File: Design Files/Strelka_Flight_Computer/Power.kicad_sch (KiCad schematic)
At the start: 41 parts, among them J1 1S_LiPo_LARGE_HOLE_XT-30, Q1 ??, Q2 ??, SW3 SW_DIP_x01, U16 TPS61085DGKR, U2 AP9101CK6, U3 AMS1117-3.3

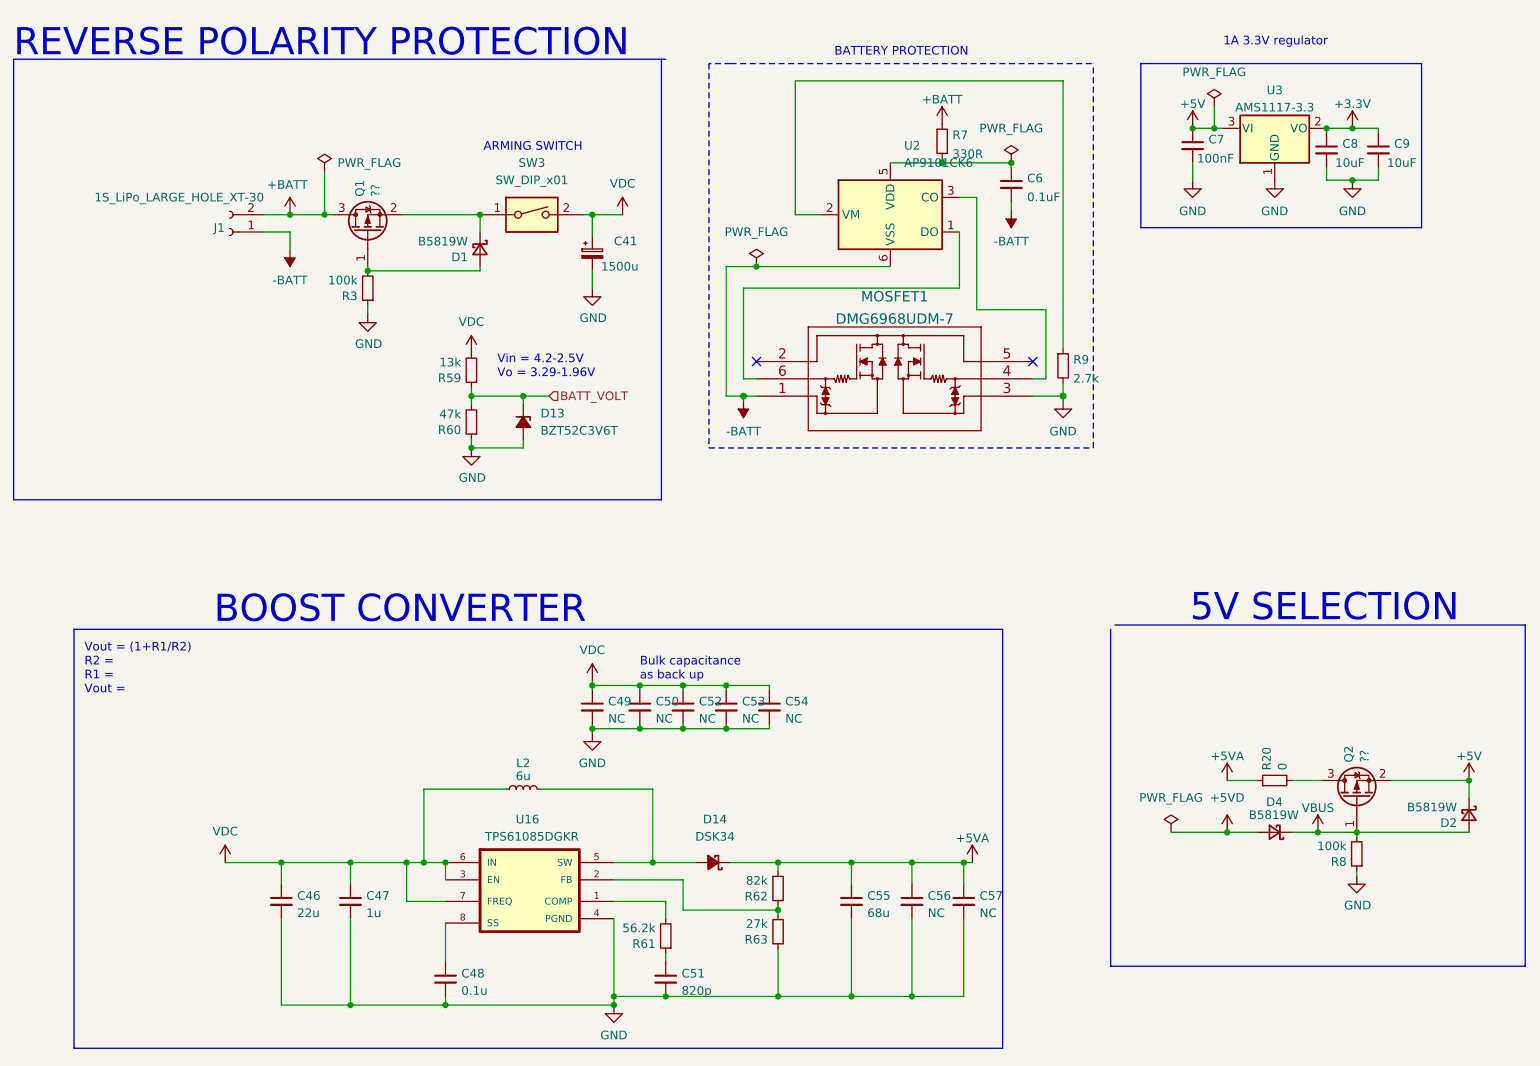
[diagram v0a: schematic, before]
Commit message: Creating BOM
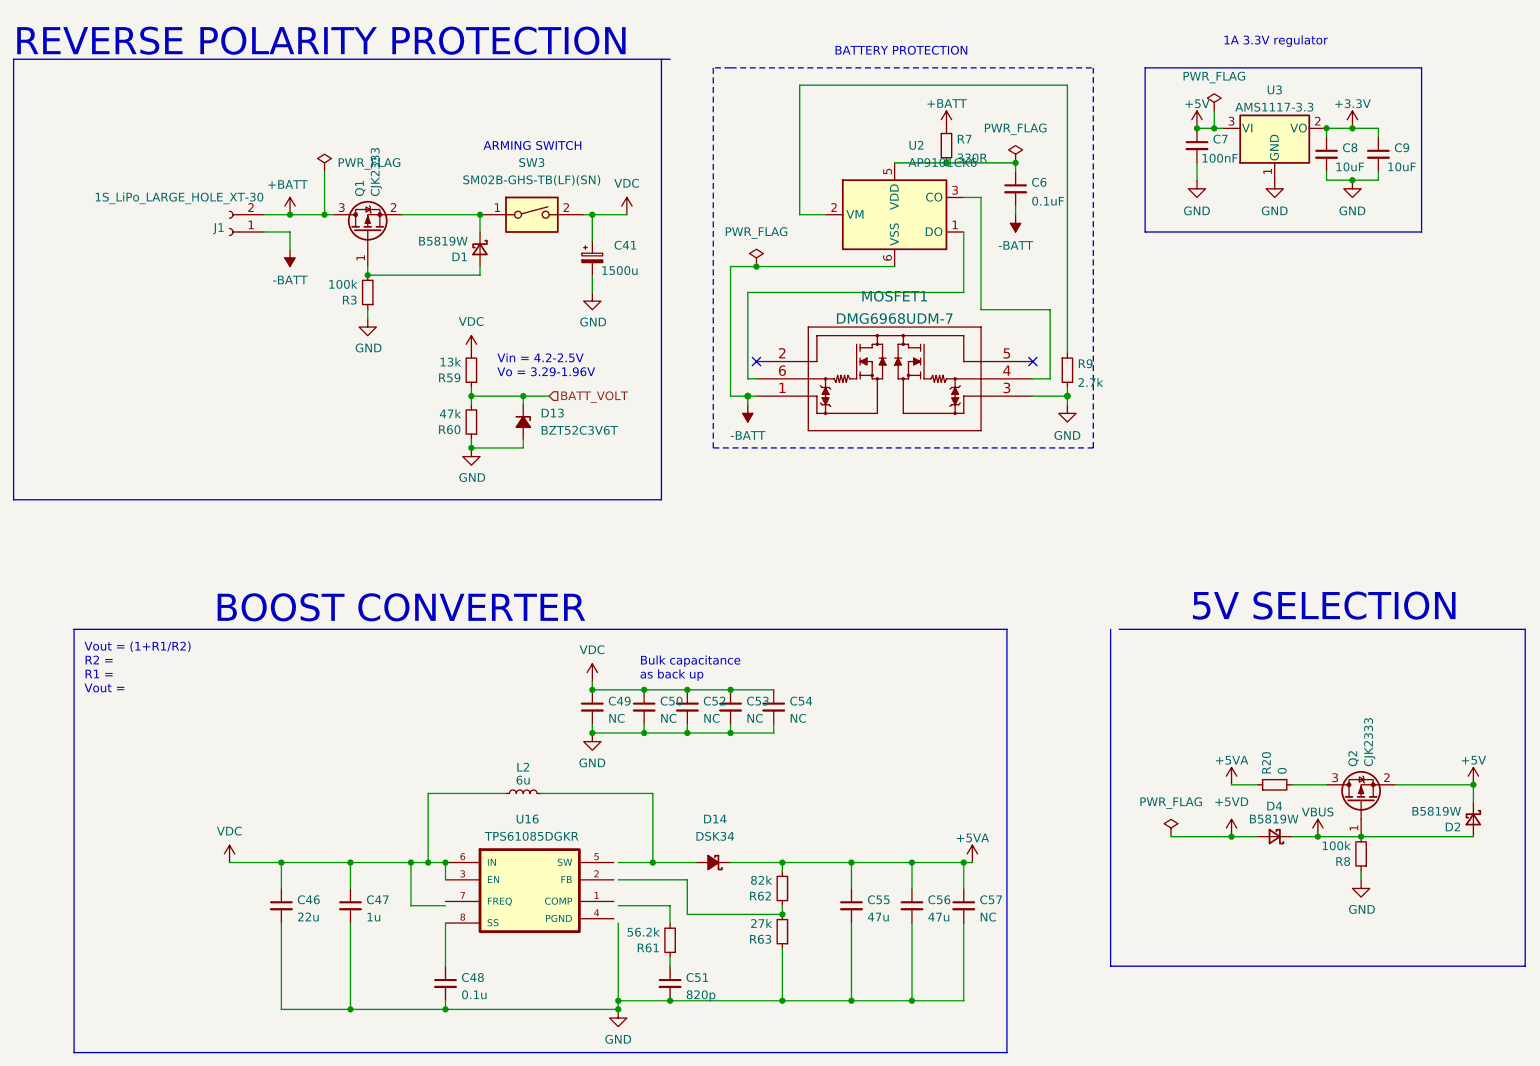
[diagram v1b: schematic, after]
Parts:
- C55: value 68u -> 47u
- C56: value NC -> 47u; footprint Capacitor_SMD:C_0603_1608Metric -> Capacitor_SMD:C_0805_2012Metric
- C57: footprint Capacitor_SMD:C_0603_1608Metric -> Capacitor_SMD:C_0805_2012Metric
- D1, D2, D4: LCSC# (none) -> C8598
- MOSFET1: LCSC# (none) -> C151635; MFR# DMG6968UDM-7 -> (none)
- Q1, Q2: value ?? -> CJK2333; LCSC# (none) -> C504109
- SW3: value SW_DIP_x01 -> SM02B-GHS-TB(LF)(SN); LCSC# (none) -> C189893
- U16: AVAILABILITY Unavailable -> (none); DESCRIPTION 18.5V, 2A, 650kHz / 1.2MHz Step-Up DC-DC Converter w/ Force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 -> (none); LCSC# (none) -> C113659; MF Texas Instruments -> (none); MOUSER-PURCHASE-URL https://snapeda.com/shop?store=Mouser&id=1236975 -> (none); MP TPS61085DGKR -> (none); PACKAGE VSSOP-8 Texas Instruments -> (none); PRICE None -> (none); TEXAS_INSTRUMENTS-PURCHASE-URL https://snapeda.com/shop?store=Texas+Instruments&id=1236975 -> (none)
- U2: LCSC# (none) -> C151339
- U3: LCSC# (none) -> C173386
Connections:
- net GND: no longer U16.4 (PGND)
- net VDC: no longer U16.7 (FREQ)
- net at R62.1, R63.2: no longer U16.2 (FB)
- net at R61.2: no longer U16.1 (COMP)
- net at D14.2 (A), L2.2: no longer U16.5 (SW)
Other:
- moved on the sheet: C41, C46, C47, C48, C50, C51, C52, C53, C54, C55, C56, C57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
